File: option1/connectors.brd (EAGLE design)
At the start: 13 x 14.5 mm, 14 parts, among them CON1 PINHEAD_1X06-2, CON2 PINHEAD_1X03-2.54-RA, CON3 CON-4P-JST_GH-RA, CON4 PINHEAD_1X02-2, CON5 PINHEAD_1X02-2, CON8 CON-4P-JST_GH-RA, IC3 TJA1051

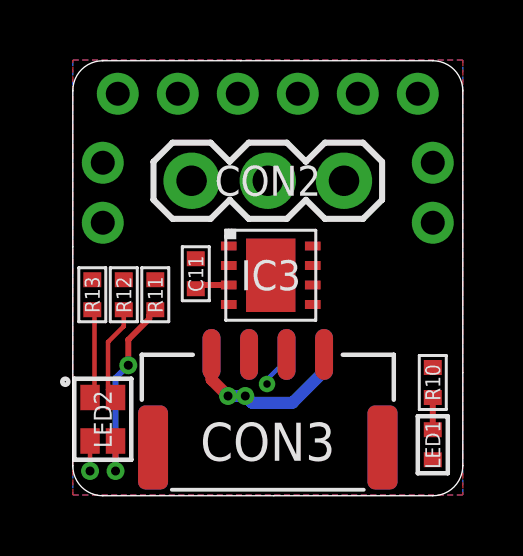
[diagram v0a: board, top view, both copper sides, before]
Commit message: updates here and there
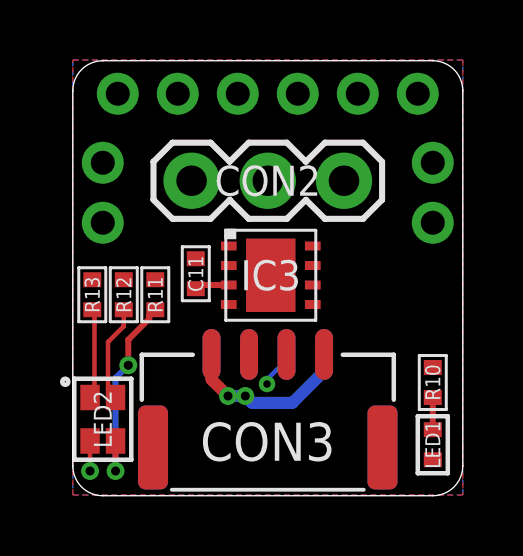
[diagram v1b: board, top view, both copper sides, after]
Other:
- outline, holes or cut-outs redrawn
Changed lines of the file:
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@@
 <setting verticaltext="up"/>
 </settings>
-<grid distance="0.05" unitdist="mm" unit="mm" style="lines" multiple="1" display="no" altdistance="5" altunitdist="mil" altunit="mil"/>
+<grid distance="0.5" unitdist="mm" unit="mm" style="lines" multiple="1" display="no" altdistance="5" altunitdist="mil" altunit="mil"/>
 <layers>
 <layer number="1" name="Top" color="4" fill="1" visible="yes" active="yes"/>
@@
 <layer number="14" name="Route14" color="22" fill="1" visible="no" active="no"/>
 <layer number="15" name="Route15" color="23" fill="1" visible="no" active="no"/>
-<layer number="16" name="Bottom" color="1" fill="1" visible="yes" active="yes"/>
-<layer number="17" name="Pads" color="2" fill="1" visible="yes" active="yes"/>
-<layer number="18" name="Vias" color="2" fill="1" visible="yes" active="yes"/>
-<layer number="19" name="Unrouted" color="6" fill="1" visible="yes" active="yes"/>
+<layer number="16" name="Bottom" color="1" fill="1" visible="no" active="yes"/>
+<layer number="17" name="Pads" color="2" fill="1" visible="no" active="yes"/>
+<layer number="18" name="Vias" color="2" fill="1" visible="no" active="yes"/>
+<layer number="19" name="Unrouted" color="6" fill="1" visible="no" active="yes"/>
 <layer number="20" name="Dimension" color="24" fill="1" visible="yes" active="yes"/>
 <layer number="21" name="tPlace" color="7" fill="1" visible="yes" active="yes"/>
-<layer number="22" name="bPlace" color="7" fill="1" visible="yes" active="yes"/>
+<layer number="22" name="bPlace" color="7" fill="1" visible="no" active="yes"/>
 <layer number="23" name="tOrigins" color="15" fill="1" visible="yes" active="yes"/>
-<layer number="24" name="bOrigins" color="15" fill="1" visible="yes" active="yes"/>
+<layer number="24" name="bOrigins" color="15" fill="1" visible="no" active="yes"/>
 <layer number="25" name="tNames" color="7" fill="1" visible="yes" active="yes"/>
-<layer number="26" name="bNames" color="7" fill="1" visible="yes" active="yes"/>
-<layer number="27" name="tValues" color="7" fill="1" visible="yes" active="yes"/>
+<layer number="26" name="bNames" color="7" fill="1" visible="no" active="yes"/>
+<layer number="27" name="tValues" color="7" fill="1" visible="no" active="yes"/>
 <layer number="28" name="bValues" color="7" fill="1" visible="no" active="yes"/>
 <layer number="29" name="tStop" color="7" fill="3" visible="no" active="yes"/>
@@
 <layer number="37" name="tTest" color="7" fill="1" visible="no" active="yes"/>
 <layer number="38" name="bTest" color="7" fill="1" visible="no" active="yes"/>
-<layer number="39" name="tKeepout" color="4" fill="11" visible="yes" active="yes"/>
+<layer number="39" name="tKeepout" color="4" fill="11" visible="no" active="yes"/>
 <layer number="40" name="bKeepout" color="1" fill="11" visible="no" active="yes"/>
-<layer number="41" name="tRestrict" color="4" fill="10" visible="yes" active="yes"/>
+<layer number="41" name="tRestrict" color="4" fill="10" visible="no" active="yes"/>
 <layer number="42" name="bRestrict" color="1" fill="10" visible="no" active="yes"/>
 <layer number="43" name="vRestrict" color="2" fill="10" visible="no" active="yes"/>
 <layer number="44" name="Drills" color="7" fill="1" visible="no" active="yes"/>
-<layer number="45" name="Holes" color="7" fill="1" visible="yes" active="yes"/>
+<layer number="45" name="Holes" color="7" fill="1" visible="no" active="yes"/>
 <layer number="46" name="Milling" color="3" fill="1" visible="no" active="yes"/>
 <layer number="47" name="Measures" color="7" fill="1" visible="no" active="yes"/>
 <layer number="48" name="Document" color="7" fill="1" visible="no" active="yes"/>
-<layer number="49" name="Reference" color="7" fill="1" visible="yes" active="yes"/>
+<layer number="49" name="Reference" color="7" fill="1" visible="no" active="yes"/>
 <layer number="50" name="dxf" color="7" fill="1" visible="no" active="no"/>
 <layer number="51" name="tDocu" color="7" fill="1" visible="yes" active="yes"/>
-<layer number="52" name="bDocu" color="7" fill="1" visible="yes" active="yes"/>
+<layer number="52" name="bDocu" color="7" fill="1" visible="no" active="yes"/>
 <layer number="53" name="tGND_GNDA" color="7" fill="9" visible="no" active="no"/>
 <layer number="54" name="bGND_GNDA" color="1" fill="9" visible="no" active="no"/>
@@
 </layers>
 <board>
-<fusionsync huburn="a.cGVyc29uYWw6dWUyYWE4ZDY4" projecturn="a.cGVyc29uYWw6dWUyYWE4ZDY4IzIwMTgxMTA3MTU4OTYxMDMx" f3durn="urn:adsk.wipprod:dm.lineage:F6T5hmtoRzyO-gJKBP2O0Q" pcbguid="9eefd93a-a020-4737-8592-dac48cb7ff18" lastpulledtime="" lastsyncedchangeguid="2dd12a48-ca80-25c8-6762-f0f654a6b96e"/>
+<fusionsync huburn="a.cGVyc29uYWw6dWUyYWE4ZDY4" projecturn="a.cGVyc29uYWw6dWUyYWE4ZDY4IzIwMTgxMTA4MTU5MTUwNTA2" f3durn="urn:adsk.wipprod:dm.lineage:W-AU7Z-WRBGsUBjO-a_i9g" pcbguid="b2c5e014-5653-4791-840d-ae12ea5a7034" lastpulledtime="2018-11-08T17:53:16Z" lastsyncedchangeguid="92847348-70cf-7b2c-bcb8-8c73375c68d2"/>
 <plain>
 <wire x1="-20" y1="0" x2="0" y2="20" width="0.01" layer="48" curve="-90"/>
@@
 <wire x1="20" y1="-20" x2="-20" y2="-20" width="0.01" layer="48"/>
 <wire x1="-20" y1="-20" x2="-20" y2="0" width="0.01" layer="48"/>
-<wire x1="0.2" y1="-2.5" x2="-5.5" y2="-2.5" width="0.01" layer="20"/>
-<wire x1="-5.5" y1="-2.5" x2="-6.5" y2="-1.5" width="0.01" layer="20" curve="-90"/>
-<wire x1="-6.5" y1="-1.5" x2="-6.5" y2="5.8" width="0.01" layer="20"/>
-<wire x1="-6.5" y1="5.8" x2="-6.5" y2="11" width="0.01" layer="20"/>
-<wire x1="-6.5" y1="11" x2="-5.5" y2="12" width="0.01" layer="20" curve="-90"/>
-<wire x1="-5.5" y1="12" x2="-0.9" y2="12" width="0.01" layer="20"/>
-<wire x1="-0.9" y1="12" x2="5.5" y2="12" width="0.01" layer="20"/>
-<wire x1="5.5" y1="12" x2="6.5" y2="11" width="0.01" layer="20" curve="-90"/>
-<wire x1="6.5" y1="11" x2="6.5" y2="1.6" width="0.01" layer="20"/>
-<wire x1="6.5" y1="1.6" x2="6.5" y2="-1.5" width="0.01" layer="20"/>
-<wire x1="6.5" y1="-1.5" x2="5.5" y2="-2.5" width="0.01" layer="20" curve="-90"/>
-<wire x1="5.5" y1="-2.5" x2="0.2" y2="-2.5" width="0.01" layer="20"/>
+<wire x1="5.5" y1="-2.5" x2="6.5" y2="-1.5" width="0.01" layer="20" curve="90"/>
+<wire x1="6.5" y1="-1.5" x2="6.5" y2="11" width="0.01" layer="20"/>
+<wire x1="6.5" y1="11" x2="5.5" y2="12" width="0.01" layer="20" curve="90"/>
+<wire x1="5.5" y1="12" x2="-5.5" y2="12" width="0.01" layer="20"/>
+<wire x1="-5.5" y1="12" x2="-6.5" y2="11" width="0.01" layer="20" curve="90"/>
+<wire x1="-6.5" y1="11" x2="-6.5" y2="-1.5" width="0.01" layer="20"/>
+<wire x1="-6.5" y1="-1.5" x2="-5.5" y2="-2.5" width="0.01" layer="20" curve="90"/>
+<wire x1="-5.5" y1="-2.5" x2="5.5" y2="-2.5" width="0.01" layer="20"/>
 </plain>
 <attributes>
